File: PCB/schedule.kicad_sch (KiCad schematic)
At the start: 7 parts, among them SW1 SW_Push, SW2 SW_Push, SW3 SW_Push, SW4 SW_Push, U1 XIAO-RP2040-DIP

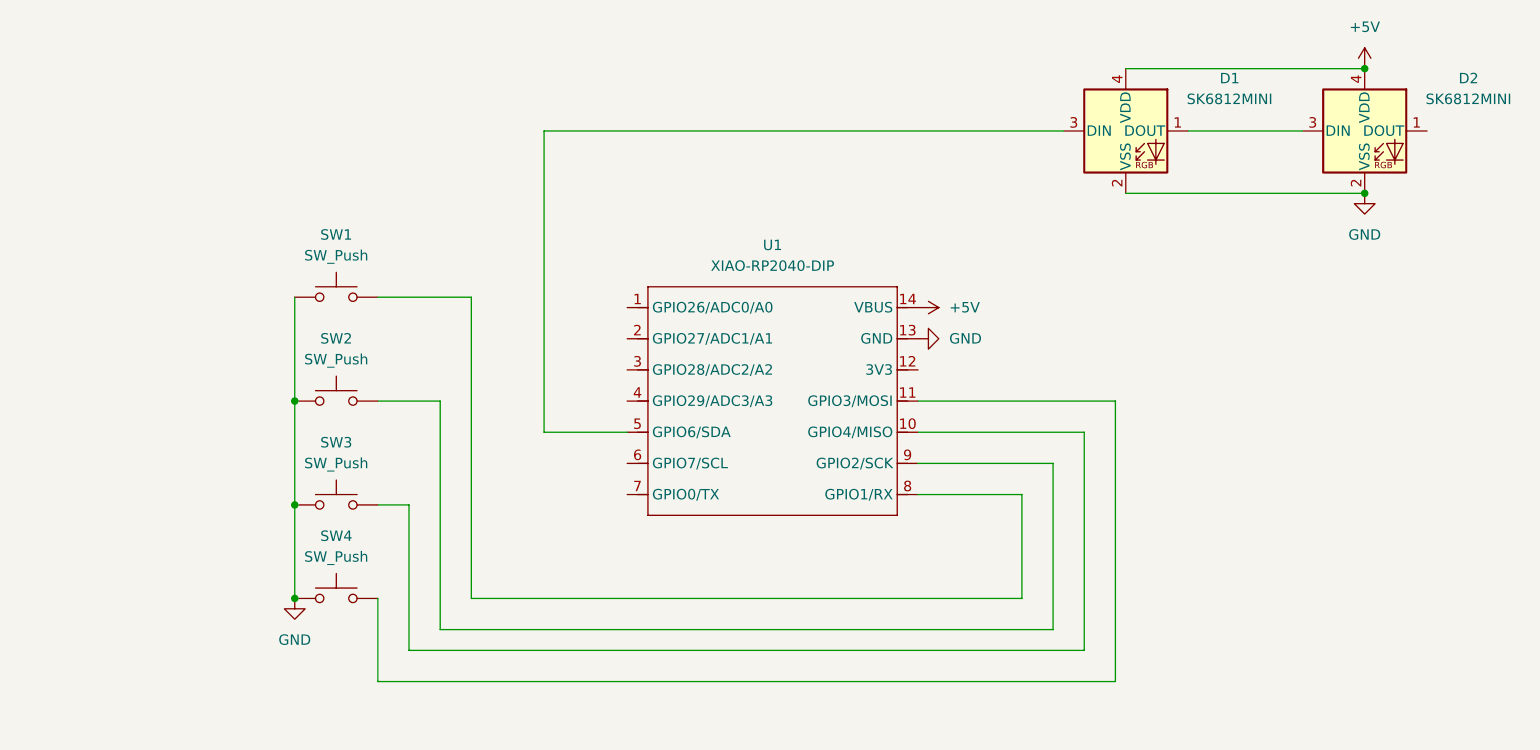
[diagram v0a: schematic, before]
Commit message: Remodelation
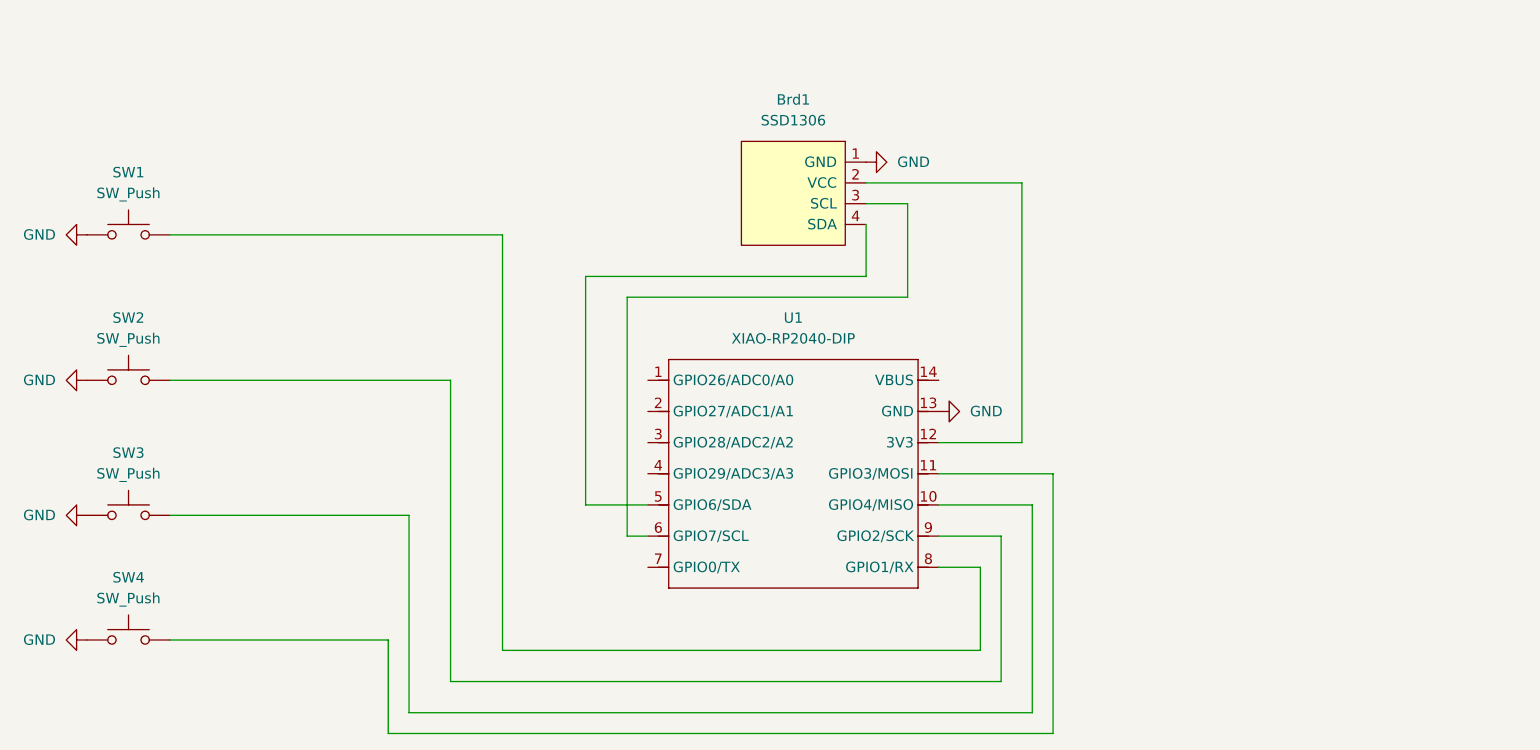
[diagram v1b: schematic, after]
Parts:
- removed D1, D2: SK6812MINI, LED_SMD:LED_SK6812MINI_PLCC4_3.5x3.5mm_P1.75mm, symbol LED:SK6812MINI
- added Brd1: SSD1306, Display:Adafruit_SSD1306, symbol SSD1306-128x64_OLED:SSD1306
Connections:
- net GND: now also Brd1.1 (GND)
- net at U1.12 (3V3): now also Brd1.2 (VCC)
- net at U1.5 (GPIO6/SDA): now also Brd1.4 (SDA)
- net at U1.6 (GPIO7/SCL): now also Brd1.3 (SCL)
- net +5V: no longer names the net of U1.14 (VBUS)
